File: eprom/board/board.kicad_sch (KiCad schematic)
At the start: 21 parts, among them J1 GPIO, J2 PWR, Q1 2N3904, Q2 BS250, U1 8755A, U2 MC33063AP

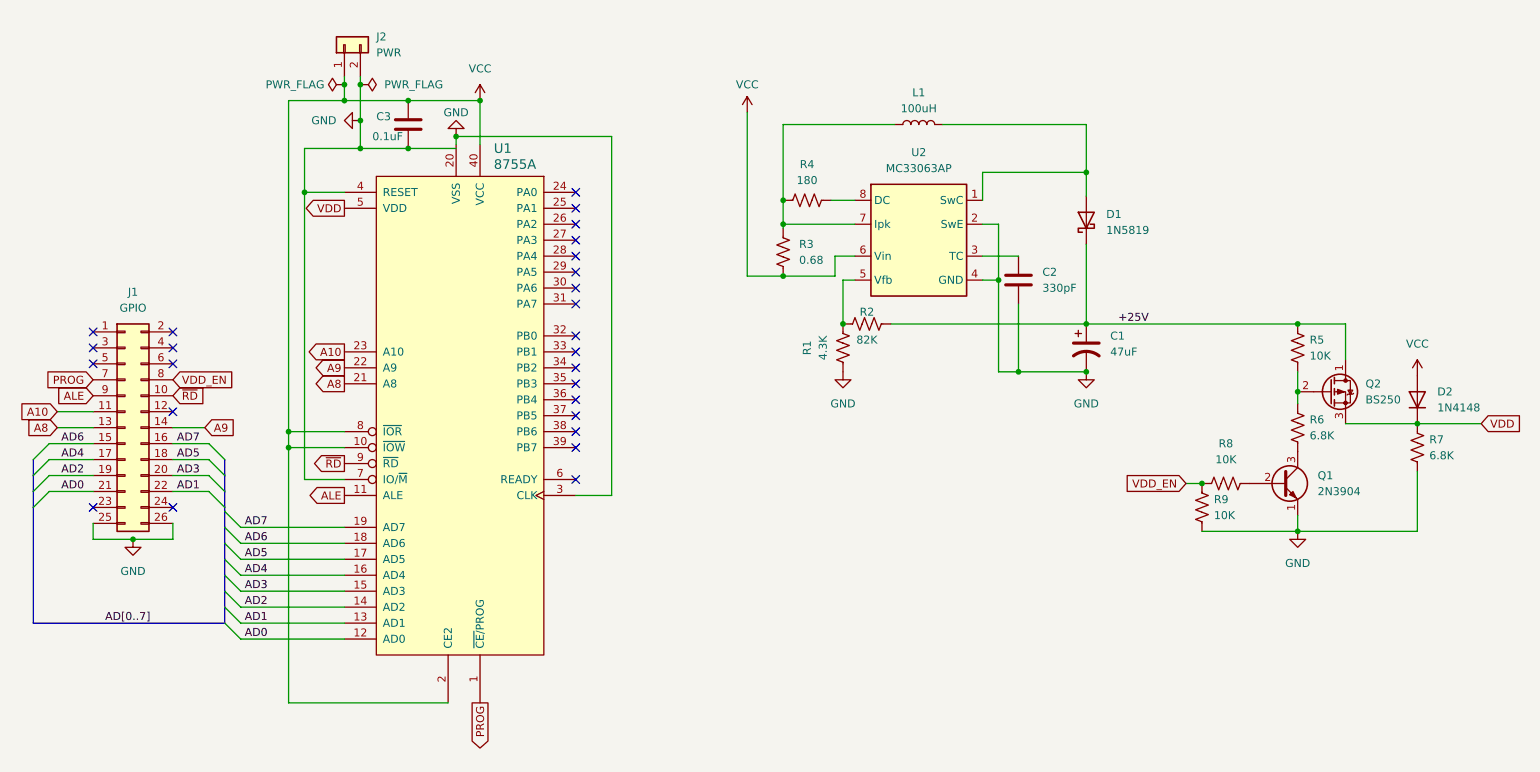
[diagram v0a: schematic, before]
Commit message: Production version
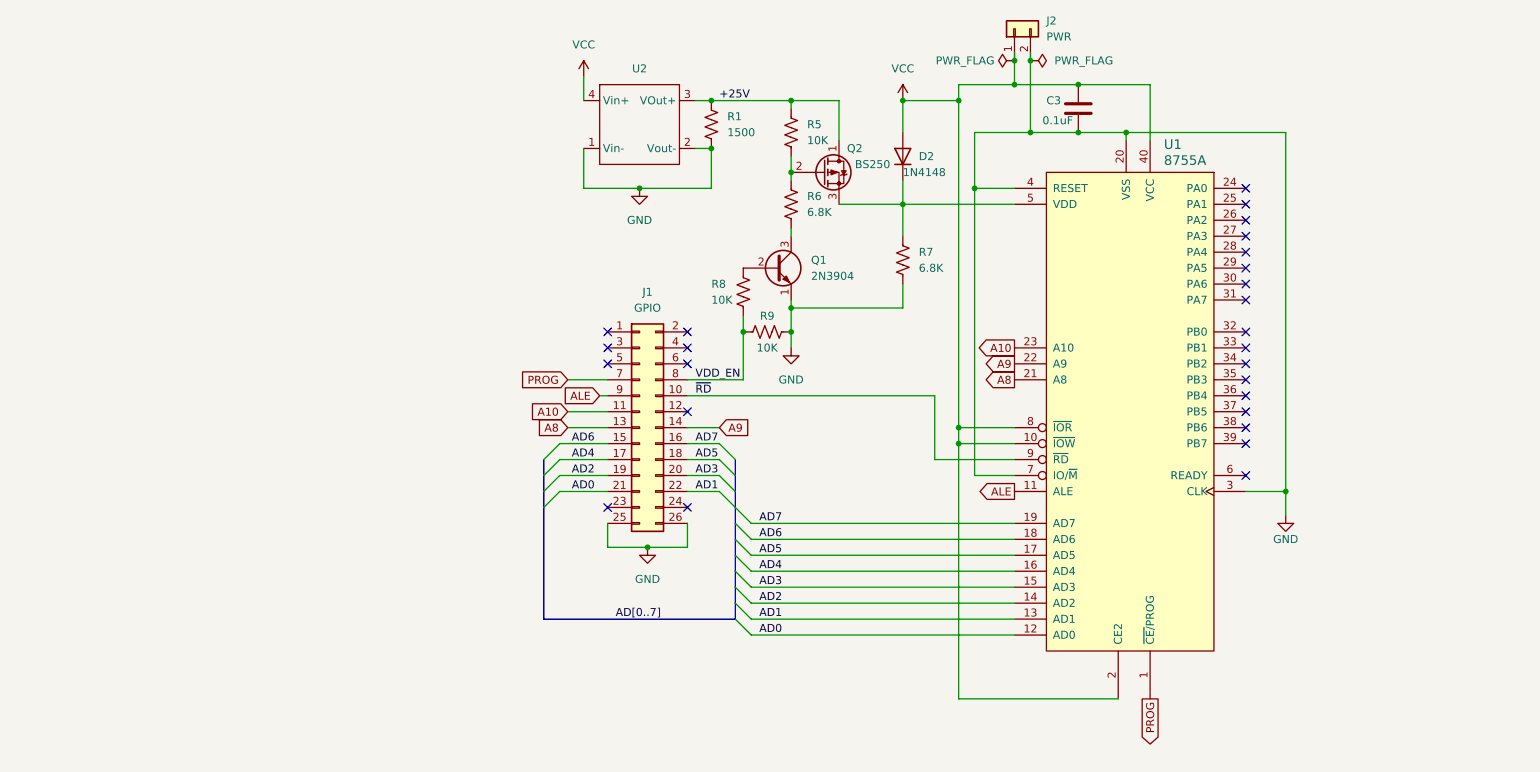
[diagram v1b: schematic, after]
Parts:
- removed C1: 47uF, Capacitor_THT:CP_Radial_Tantal_D4.5mm_P2.50mm, symbol Device:C_Polarized_US
- removed C2: 330pF, Capacitor_THT:C_Disc_D7.5mm_W4.4mm_P5.00mm, symbol Device:C
- removed D1: 1N5819, Diode_THT:D_DO-41_SOD81_P7.62mm_Horizontal, symbol Device:D_Schottky
- removed L1: 100uH, Inductor_THT:L_Radial_D7.0mm_P3.00mm, symbol Device:L
- removed R2: 82K, Resistor_THT:R_Axial_DIN0207_L6.3mm_D2.5mm_P10.16mm_Horizontal, symbol Device:R_US
- removed R3: 0.68, Resistor_THT:R_Axial_DIN0207_L6.3mm_D2.5mm_P10.16mm_Horizontal, symbol Device:R_US
- removed R4: 180, Resistor_THT:R_Axial_DIN0207_L6.3mm_D2.5mm_P10.16mm_Horizontal, symbol Device:R_US
- removed U2: MC33063AP, Package_DIP:DIP-8_W7.62mm_Socket, symbol Regulator_Switching:MC33063AP
- added U2: ~, parts:MT3608_Module, symbol parts:MT3608_Module
- C3: footprint Capacitor_THT:C_Disc_D7.5mm_W4.4mm_P5.00mm -> Capacitor_THT:C_Disc_D9.0mm_W2.5mm_P5.00mm
- R1: value 4.3K -> 1500
- U1: footprint Package_DIP:DIP-40_W15.24mm_Socket -> Socket:3M_Textool_240-1288-00-0602J_2x20_P2.54mm
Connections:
- net +25V: now also R1.2, R5.2, U2.3 (VOut+); no longer R5.1
- net GND: now also R7.1, U2.1 (Vin-), U2.2 (Vout-); no longer R7.2
- net VCC: now also U2.4 (Vin+)
- net at Q1.3 (C): now also R6.1; no longer R6.2
- net VDD: no longer names the net of D2.1 (K), Q2.3 (S), U1.5 (VDD)
- net VDD: now also R7.2; no longer R7.1
- new net: Q2.2 (G), R5.1, R6.2
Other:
- moved on the sheet: C3, D2, J1, J2, Q1, Q2, R5, R6, R7, R8, R9, U1
